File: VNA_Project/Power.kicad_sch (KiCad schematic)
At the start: 40 parts, among them J1 Jack-DC, J201 USB_C_Receptacle_USB2.0_16P, SW1 SW_SPDT, U10 MCP1804x-A002xOT, U11 AP7375-50SA-7, U202 USBLC6-2SC6, U204 HT7533-1, U6 MIC5501-3.0YM5, U9 AP63203WU

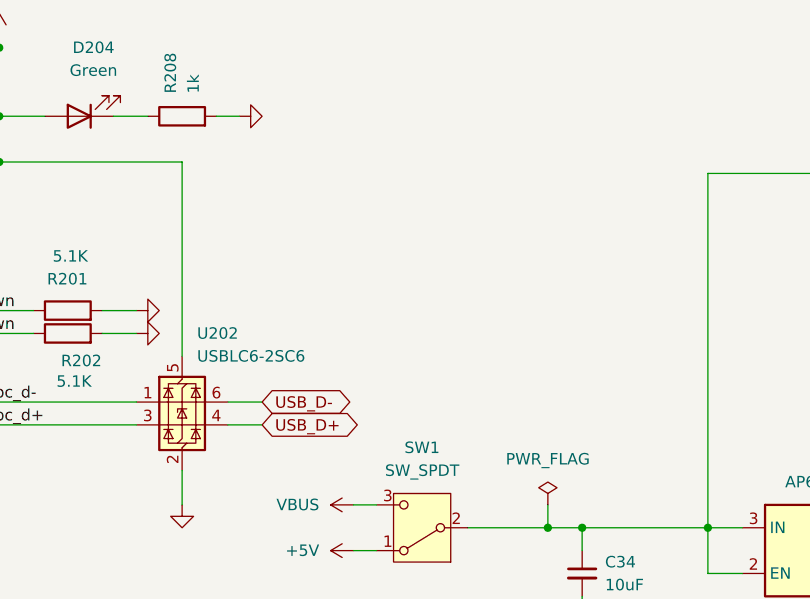
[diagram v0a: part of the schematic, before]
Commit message: AA filtering
redoing AA filtering
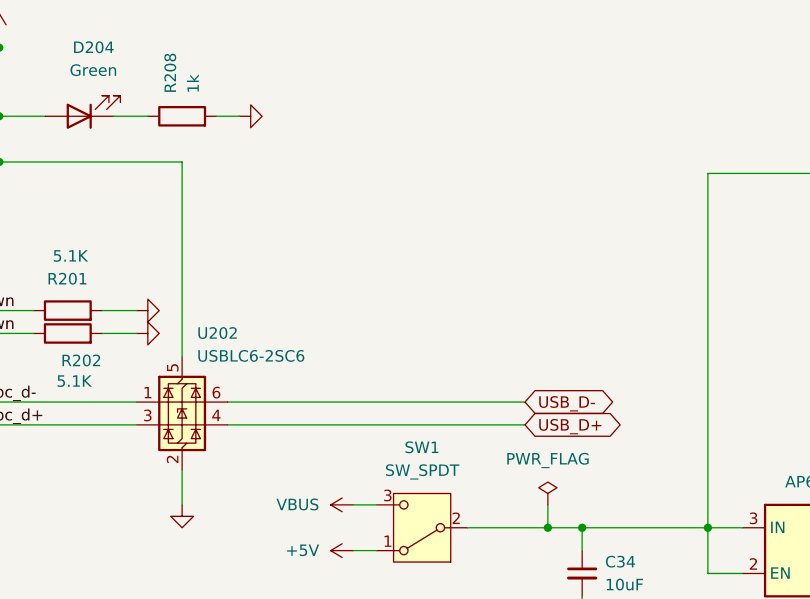
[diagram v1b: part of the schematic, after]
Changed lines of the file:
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@@
 	(wire
 		(pts
-			(xy 96.52 129.54) (xy 100.33 129.54)
+			(xy 96.52 129.54) (xy 129.54 129.54)
 		)
 		(stroke
@@
 	(wire
 		(pts
-			(xy 96.52 127) (xy 100.33 127)
+			(xy 96.52 127) (xy 129.54 127)
 		)
 		(stroke
@@
 	(wire
 		(pts
-			(xy 91.44 121.92) (xy 91.44 100.33)
+			(xy 91.44 100.33) (xy 91.44 121.92)
 		)
 		(stroke
@@
 	(global_label "USB_D-"
 		(shape bidirectional)
-		(at 100.33 127 0)
+		(at 129.54 127 0)
 		(fields_autoplaced yes)
 		(effects
@@
 		)
 		(property "Intersheetrefs" "${INTERSHEET_REFS}"
-			(at 112.0465 127 0)
+			(at 141.2565 127 0)
 			(effects
 				(font
@@
 	(global_label "USB_D+"
 		(shape bidirectional)
-		(at 100.33 129.54 0)
+		(at 129.54 129.54 0)
 		(fields_autoplaced yes)
 		(effects
@@
 		)
 		(property "Intersheetrefs" "${INTERSHEET_REFS}"
-			(at 112.0465 129.54 0)
+			(at 141.2565 129.54 0)
 			(effects
 				(font
